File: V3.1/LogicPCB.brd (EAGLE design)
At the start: 171.9 x 151.6 mm, 77 parts, among them CON1 CUBE_ORANGE_, CON10 PINHEAD_1X02-2.54, CON11 CON-4P-JST-XA, CON12 PINHEAD_1X06-2.54, CON13 CON-6P-JST-XA, CON14 PINHEAD_1X04-2.54, CON15 CON-4P-JST-XA, CON17 CON-4P-JST-XA, CON18 CON-6P-JST-XA, CON19 USB-TYPE-C-VERT-PROD, CON2 CON-4P-JST-XA, CON20 PINHEAD_1X06-2.54, CON21 CON-4P-JST-XA, CON22 CON-4P-JST-XA, CON23 CON-4P-JST-XA, CON24 CON-4P-JST-XA, CON25 CON-4P-JST-XA, CON26 CON-4P-JST-XA, CON27 CON-4P-JST-XA, CON28 CON-4P-JST-XA, CON29 CON-4P-JST-XA, CON3 RJ45-NO_SHIELD-5556416-1, CON30 CON-4P-JST-XA, CON32 CON-4P-JST-XA, CON35 CON-12P-JST-XA, CON4 CON-2P-JST-XA, CON5 CON-6P-JST-XA, CON6 CON-4P-JST-XA, CON7 PINHEAD_1X06-2.54, CON9 PINHEAD_1X12-2.54, IC5 AOZ1280, M1 05G_ETHERNET_SWITCH, Q1 IRLML0030, T1 H1102NL, T2 H1102NL, T3 H1102NL, T4 H1102NL

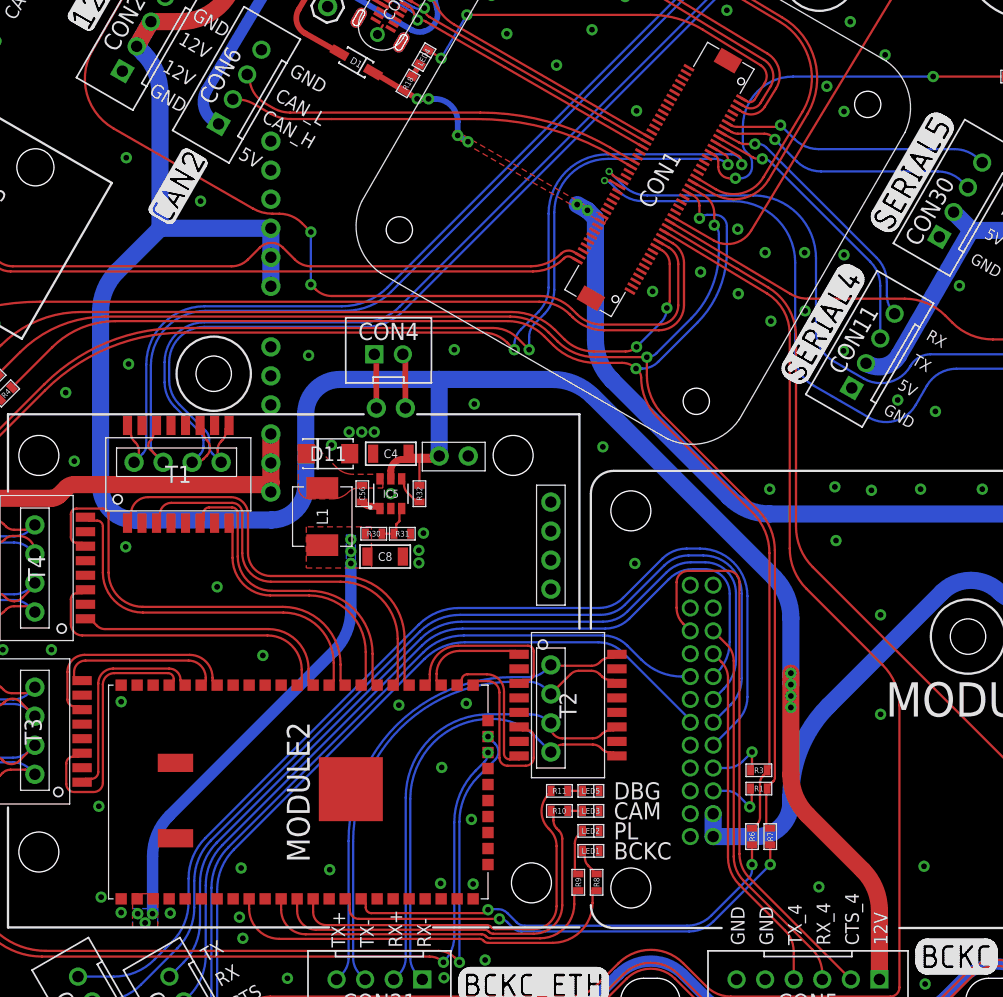
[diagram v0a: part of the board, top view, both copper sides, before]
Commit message: Naming
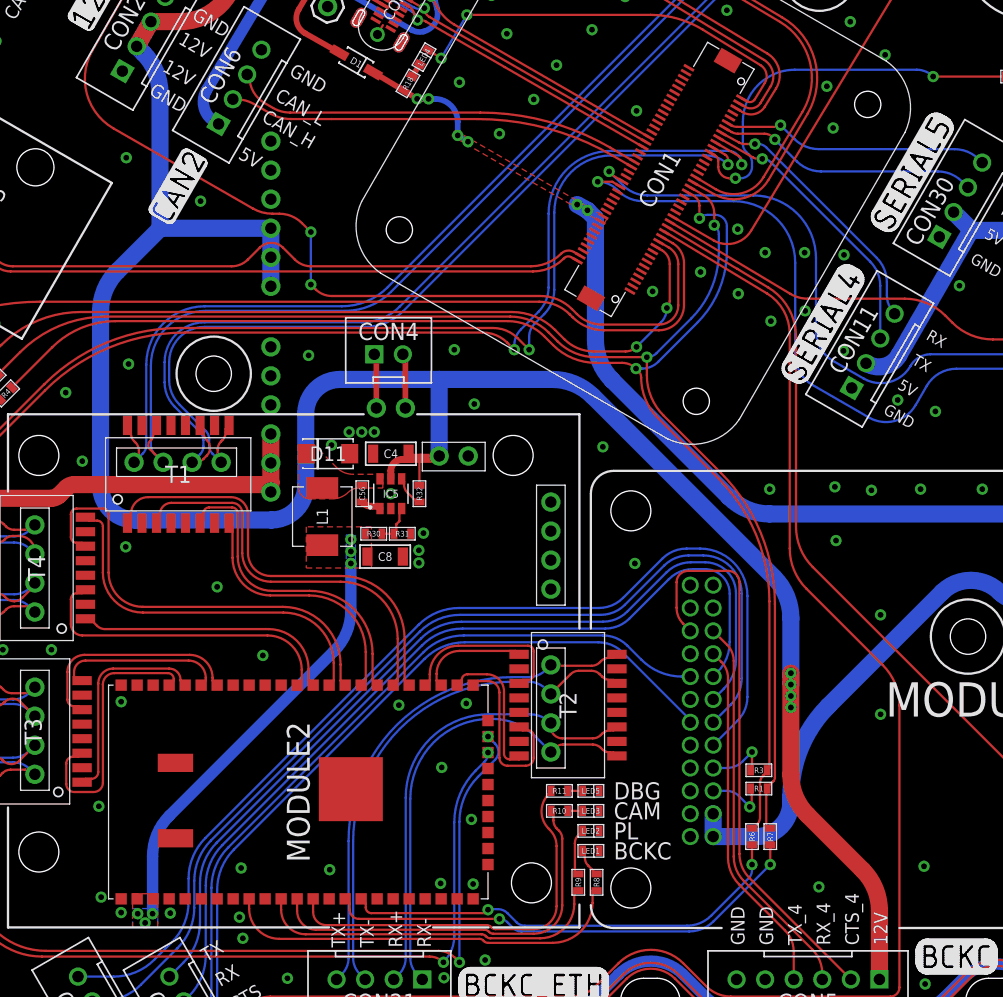
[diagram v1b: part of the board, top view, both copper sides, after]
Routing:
- net BATT_CURRENT: track 54.9 -> 56.0 mm
- net SERIAL1_RX: track 123.1 -> 122.4 mm
- net SERIAL1_TX: track 124.0 -> 123.3 mm
- net ALARM: track 33.9 -> 34.5 mm
- net GND: vias 123 -> 126

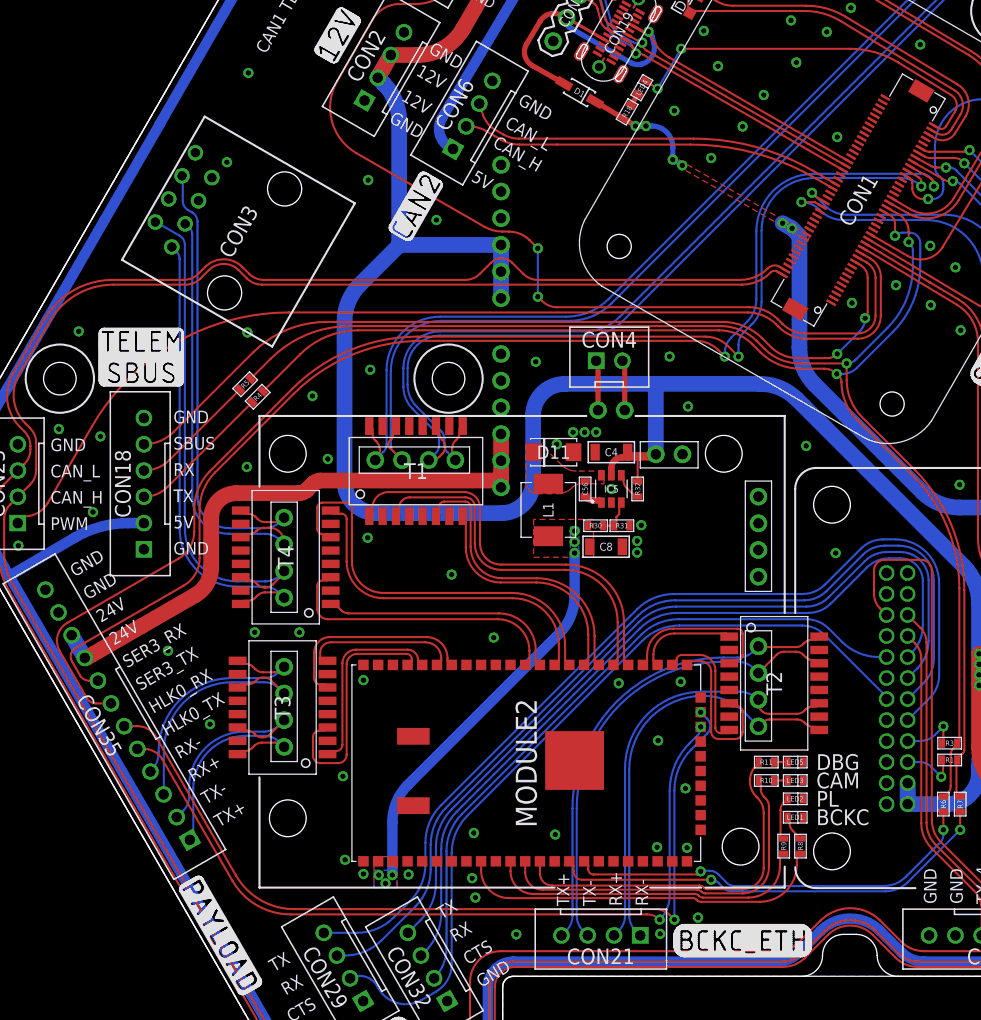
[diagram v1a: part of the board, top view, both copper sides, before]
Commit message: attribute updates
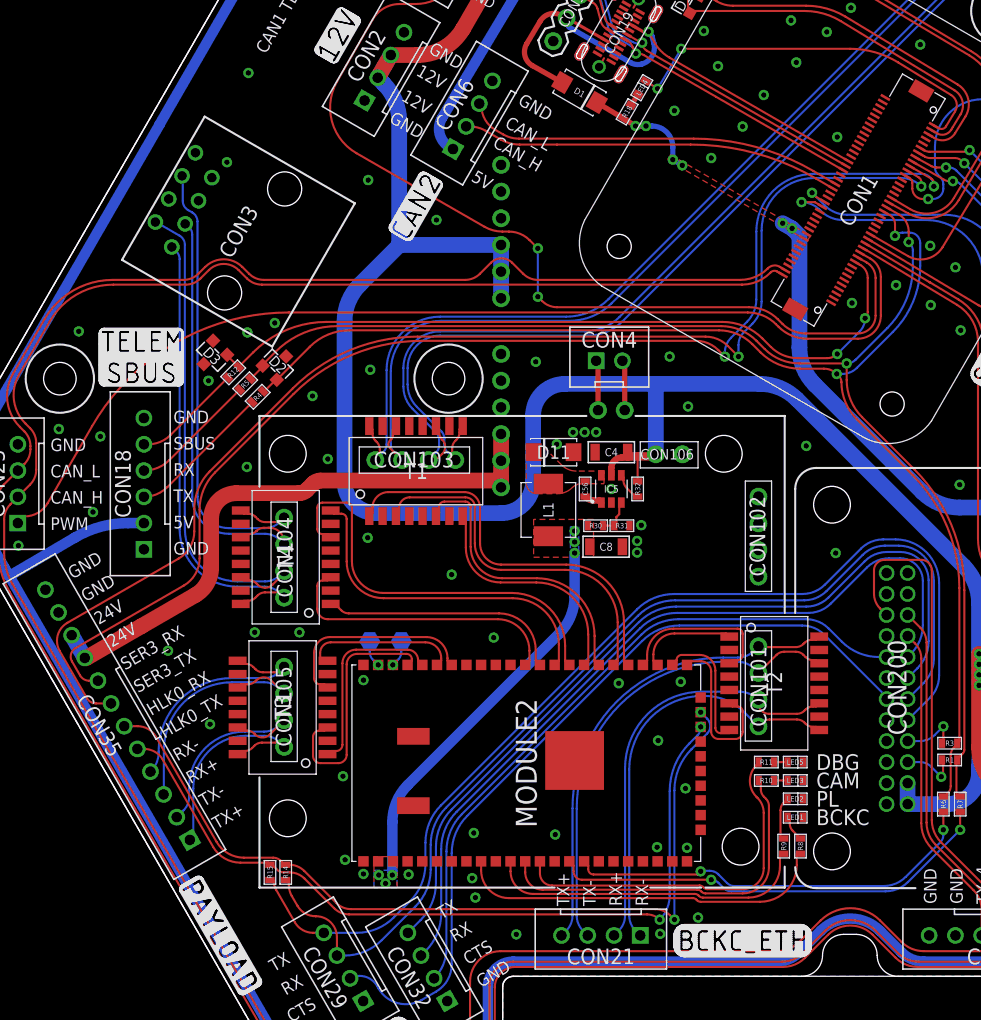
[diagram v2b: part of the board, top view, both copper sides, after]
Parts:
- added D2, D3: ESDA5V3L, TVS_diodes:SOT23B-3
- added PAD1, PAD2: PAD-HEX-2MM, PADS:HEX-2MM
- added R12, R14, R15: 120R, rc:R0603
- D1: value MBR0520L-SOD123 -> SS34; device Diodes:SOD123 -> Diodes:DO-214AC(SMA)
- R1, R3, R6, R7: value 000 -> 120R
- R10, R11, R8, R9: value (none) -> 1K
- R16: value 10K -> 51K
- R20: value 200R -> 120R
- R35, R36, R37, R38: value 100R -> 120R
- R4, R5: value (none) -> 120R
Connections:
- new net N$18: CON18.5, R12.1
- net GND: now also D2.3, D3.3
- net HLK_RX0: now also R14.1
- net HLK_TX0: now also R15.1
- net PPM-SBUS-PROT: now also D3.1, R12.2; no longer CON18.5
- net RX_2: now also R14.2
- net SERIAL1_RX: now also D2.1
- net SERIAL1_TX: now also D2.2
- net TX_2: now also R15.2
- net USB_DM: now also PAD2.1
- net USB_DP: now also PAD1.1
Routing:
- net N$18: track 0.00 -> 10.4 mm
- net PPM-SBUS-PROT: track 81.2 -> 71.0 mm
- net RX_2: track 88.6 -> 98.1 mm
- net TX_2: track 91.9 -> 99.8 mm
- net USB_DP: track 0.00 -> 2.52 mm, vias 0 -> 1
- net USB_DM: track 0.00 -> 2.52 mm, vias 0 -> 1
- net HLK_TX0: track 76.9 -> 76.3 mm
- net HLK_RX0: track 82.4 -> 81.8 mm
- net GND: vias 126 -> 128
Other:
- board text added: "CON200"
